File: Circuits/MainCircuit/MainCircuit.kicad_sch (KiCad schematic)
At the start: 42 parts, among them M1 621950 Vibration Motor, M2 FS90 Micro Servo, Q1 LTH-301-05, Q2 2N7000, Q3 2N7000, Q4 2N7000, Q5 2N7000, SW1 Reset, SW2 Tweezers, U1 PIC32MX170F256B, U2 74xxx244, U3 LED_Matrix, U4 MCP6294

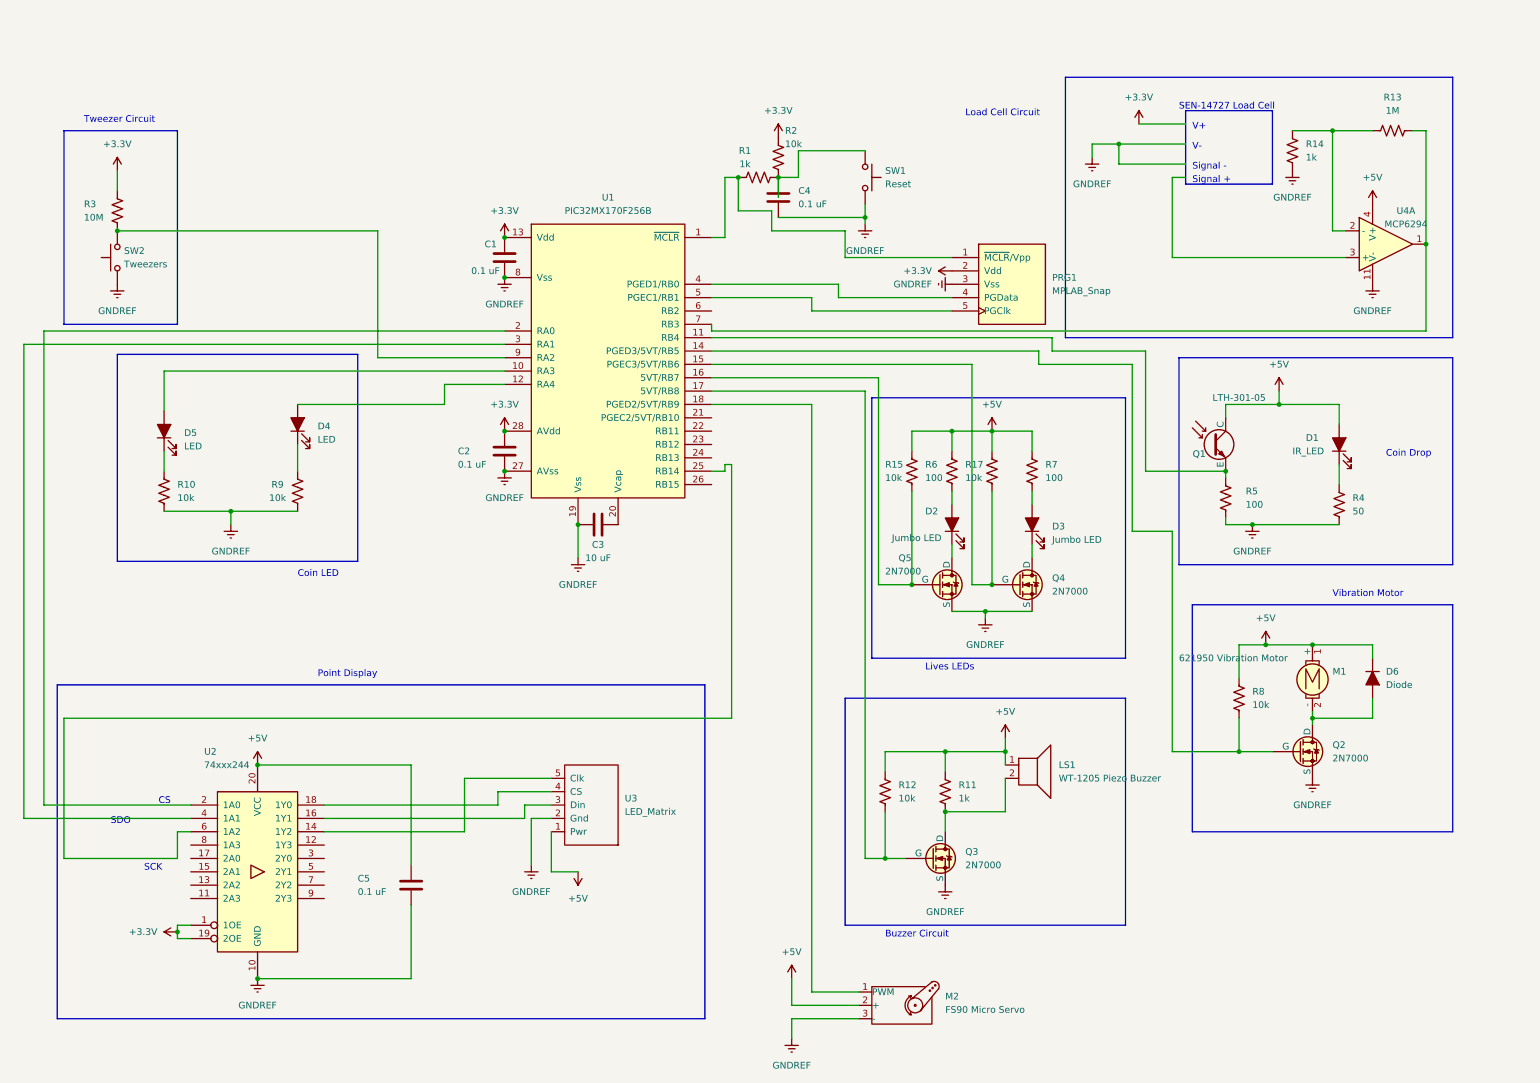
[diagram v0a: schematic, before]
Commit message: Updated KiCad With Final Circuit
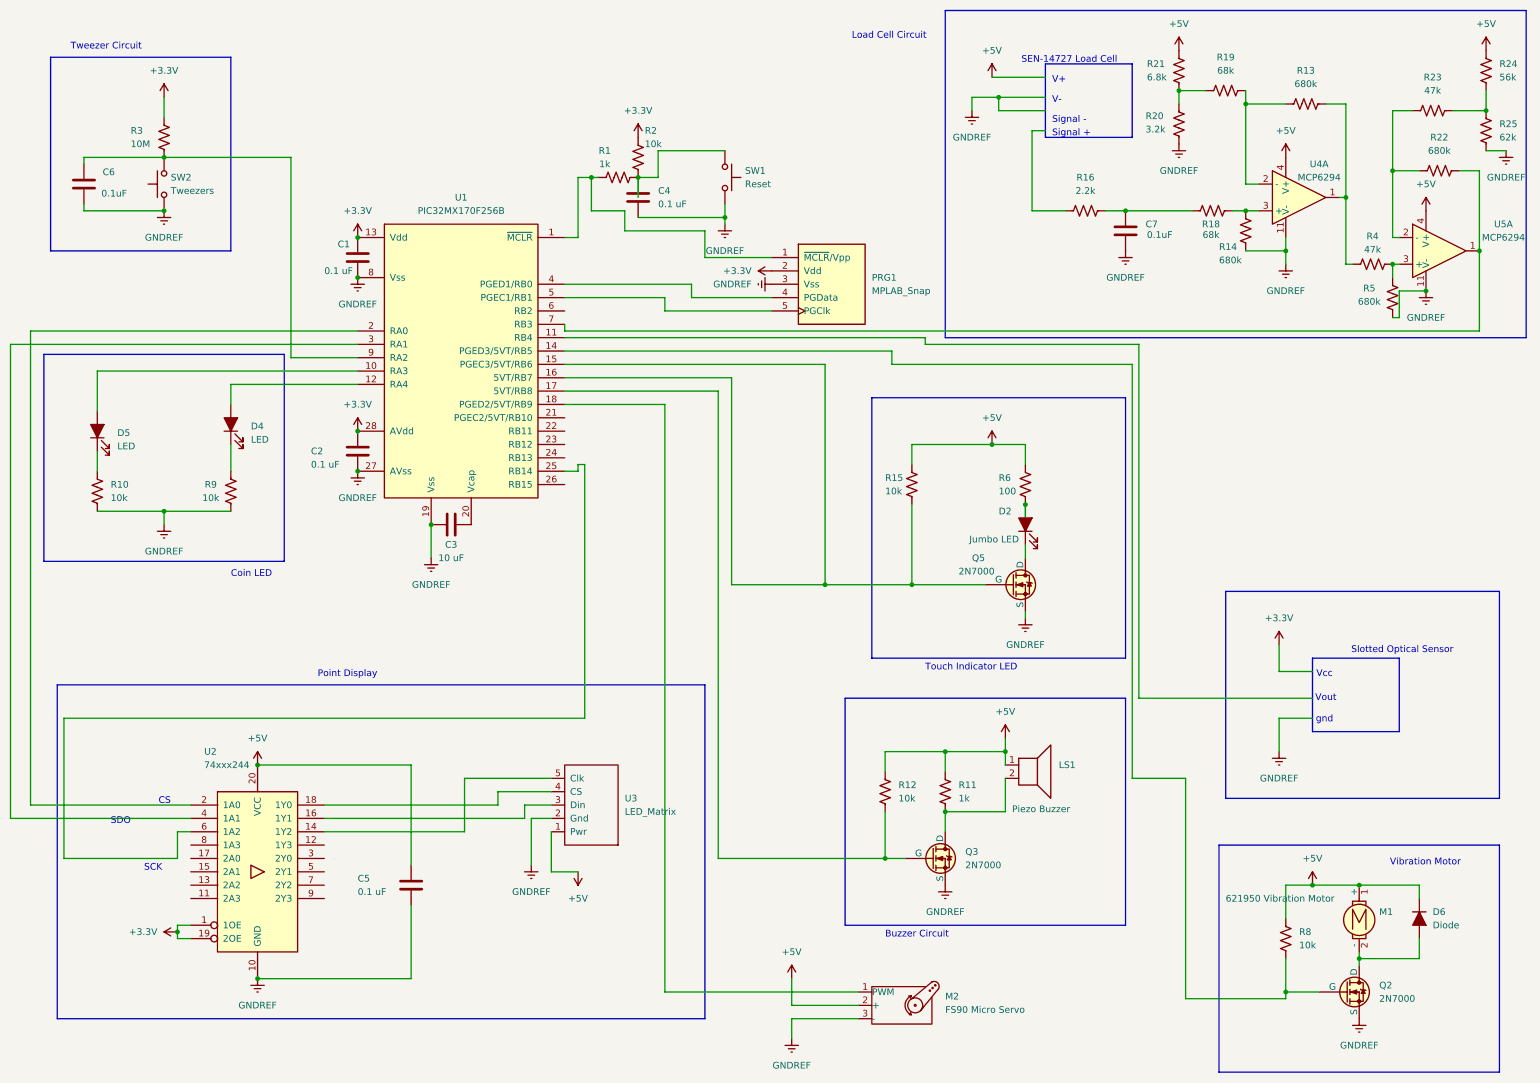
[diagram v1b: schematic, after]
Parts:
- removed D1: IR_LED, symbol ME218_BaseLib:LED
- removed D3: Jumbo LED, symbol ME218_BaseLib:LED
- removed Q1: LTH-301-05, symbol ME218_BaseLib:Photo_NPN
- removed Q4: 2N7000, symbol ME218_BaseLib:MOSFET-N
- removed R17: 10k, symbol ME218_BaseLib:Res1
- removed R7: 100, symbol ME218_BaseLib:Res1
- added C6, C7: 0.1uF, symbol ME218_BaseLib:Cap
- added R16: 2.2k, symbol ME218_BaseLib:Res1
- added R18, R19: 68k, symbol ME218_BaseLib:Res1
- added R20: 3.2k, symbol ME218_BaseLib:Res1
- added R21: 6.8k, symbol ME218_BaseLib:Res1
- added R22: 680k, symbol ME218_BaseLib:Res1
- added R23: 47k, symbol ME218_BaseLib:Res1
- added R24: 56k, symbol ME218_BaseLib:Res1
- added R25: 62k, symbol ME218_BaseLib:Res1
- added U5: MCP6294, symbol ME218_BaseLib:MCP6294
- LS1: value WT-1205 Piezo Buzzer -> Piezo Buzzer
- R13: value 1M -> 680k
- R14: value 1k -> 680k
- R4: value 50 -> 47k
- R5: value 100 -> 680k
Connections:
- net +5V: now also R21.2, R24.2, U5.4 (V+)
- net GNDREF: now also R14.1, R5.1, C6.2, C7.2, R20.1, R25.2, U5.11 (V-); no longer R14.2, R4.2, R5.2
- net at R13.2, U4.1: now also R4.1; no longer U1.7 (RB3)
- net at R13.1, U4.2 (-): now also R19.2; no longer R14.1
- net at U4.3 (+): now also R14.2, R18.2
- net at Q5.2 (G), R15.1, U1.16 (5VT/RB7): now also U1.15 (PGEC3/5VT/RB6)
- net at U1.11 (RB4): no longer R5.1
- net at R3.2, SW2.2, U1.9 (RA2): now also C6.1
- new net: C7.1, R16.2, R18.1
- new net: R22.2, U1.7 (RB3), U5.1
- new net: R22.1, R23.1, U5.2 (-)
- new net: R4.2, R5.2, U5.3 (+)
- new net: R19.1, R20.2, R21.1
- new net: R23.2, R24.1, R25.1
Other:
- note added: "Slotted Optical Sensor"
- note added: "Touch Indicator LED"
- note added: "Vcc"
- note added: "Vout"
- note added: "gnd"
- note removed: "Coin Drop"
- note removed: "Lives LEDs"
- moved on the sheet: C1, C2, C3, C4, D2, D4, D5, D6, M1, PRG1, Q2, Q5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
